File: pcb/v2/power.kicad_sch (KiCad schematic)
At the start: 72 parts, among them J16 TestPoint, J17 TestPoint, J4 Conn_01x02, J5 TestPoint, J6 TestPoint, J7 Conn_01x02, J8 Conn_01x02, J9 TestPoint, Q1 NPN, Q2 PMOS, U15 LP5907MFX-3.3, U2 TPS61230DRC, U3 LM27762, U4 TLV6213x, U5 BQ25895RTW

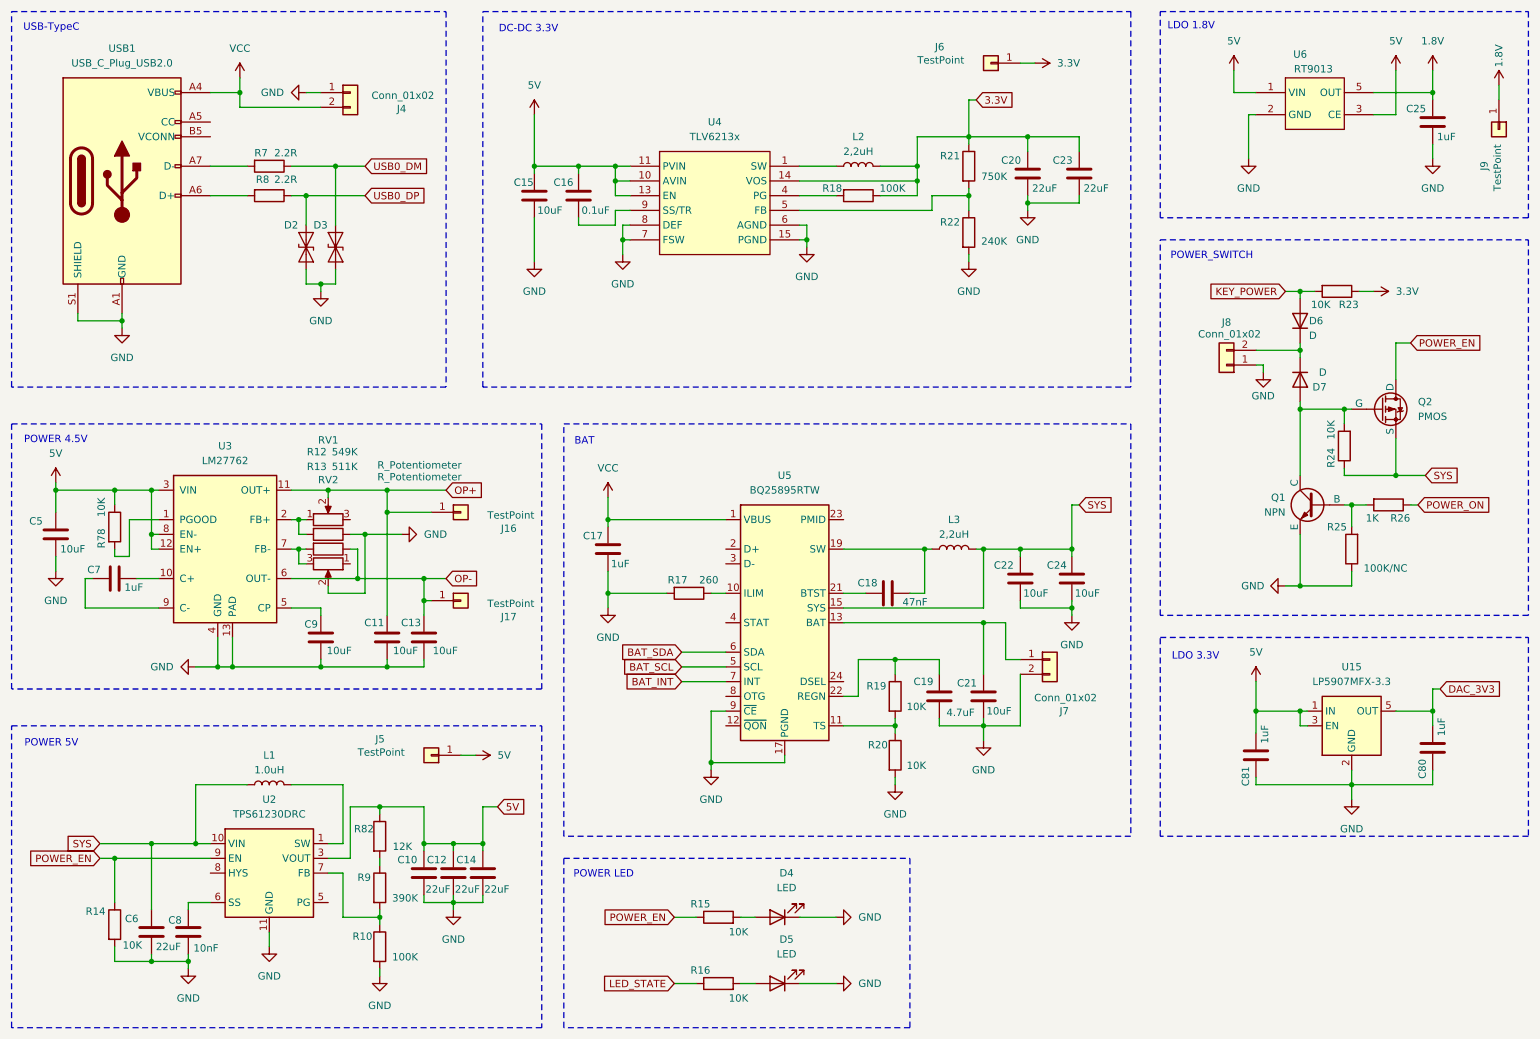
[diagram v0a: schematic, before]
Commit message: up
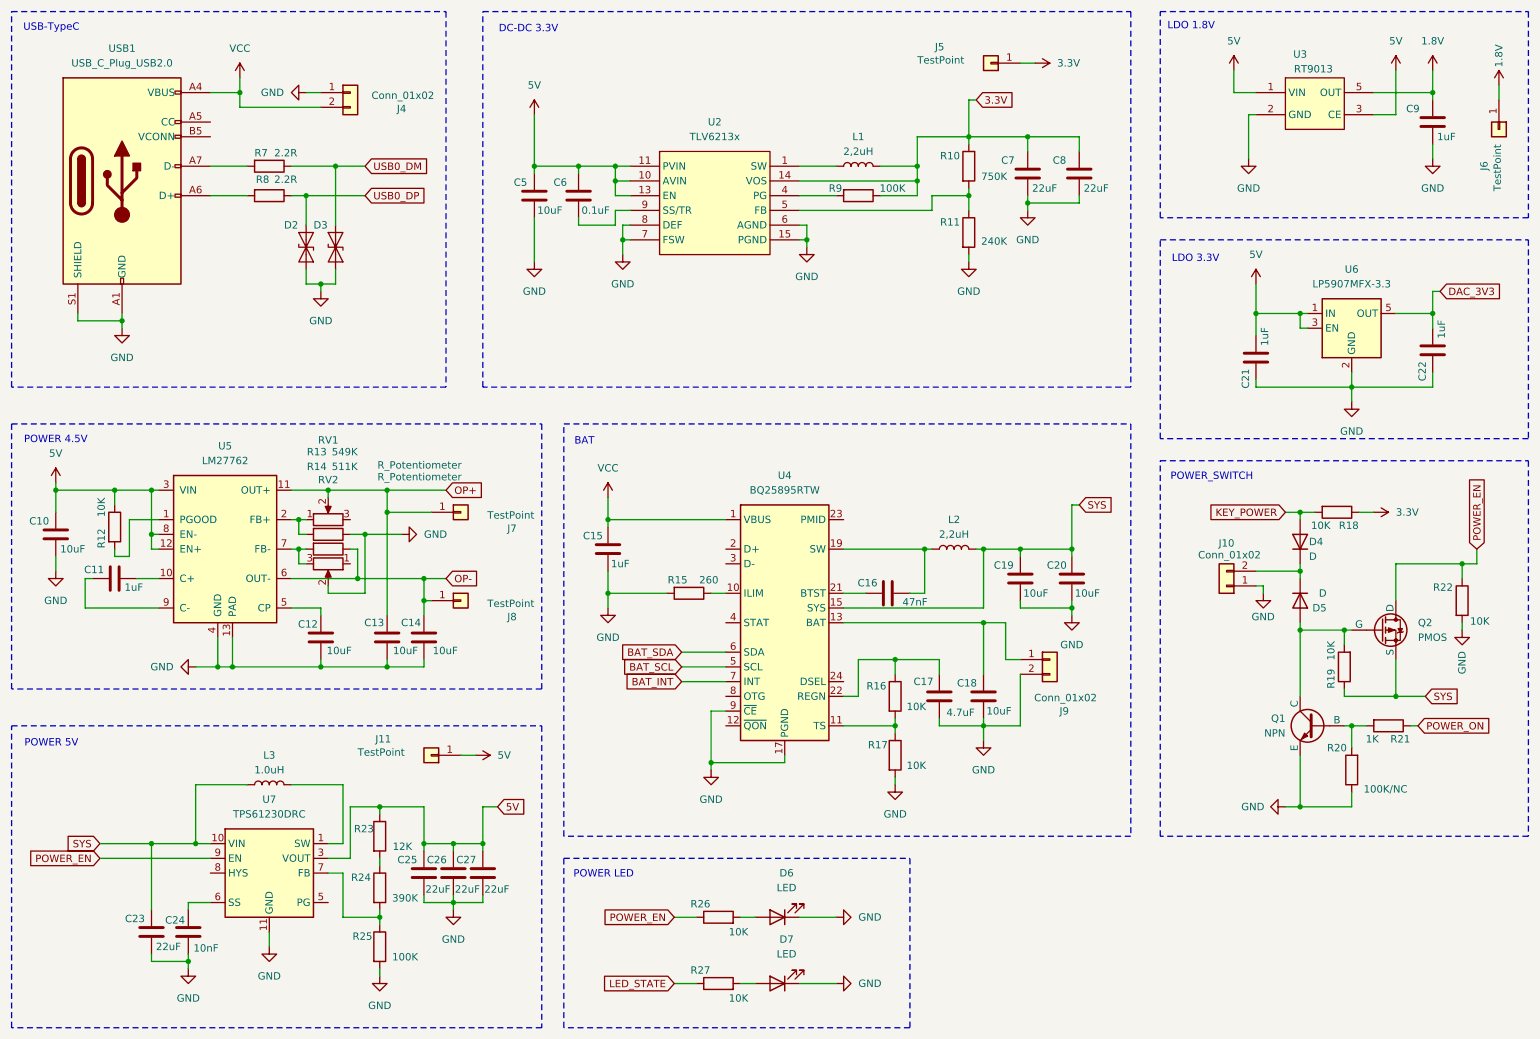
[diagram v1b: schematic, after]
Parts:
- renumbered C5 to C10, C7 to C11, C9 to C12, C11 to C13, C13 to C14, C17 to C15, C18 to C16, C19 to C17, C21 to C18, C22 to C19, C24 to C20, C81 to C21, C80 to C22, C6 to C23, C8 to C24, C10 to C25, C12 to C26, C14 to C27, C15 to C5, C16 to C6, C20 to C7, C23 to C8, C25 to C9, D6 to D4, D7 to D5, D4 to D6, D5 to D7, J8 to J10, J5 to J11, J6 to J5, J9 to J6, J16 to J7, J17 to J8, J7 to J9, L2 to L1, L3 to L2, L1 to L3, R21 to R10, R22 to R11, R78 to R12, R12 to R13, R13 to R14, R17 to R15, R19 to R16, R20 to R17, R23 to R18, R24 to R19, R25 to R20, R26 to R21, R14 to R22, R82 to R23, R9 to R24, R10 to R25, R15 to R26, R16 to R27, R18 to R9, U4 to U2, U6 to U3, U5 to U4, U3 to U5, U15 to U6, U2 to U7
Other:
- moved on the sheet: C21, C22, D4, D5, J10, Q1, Q2, R18, R19, R20, R21, R22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

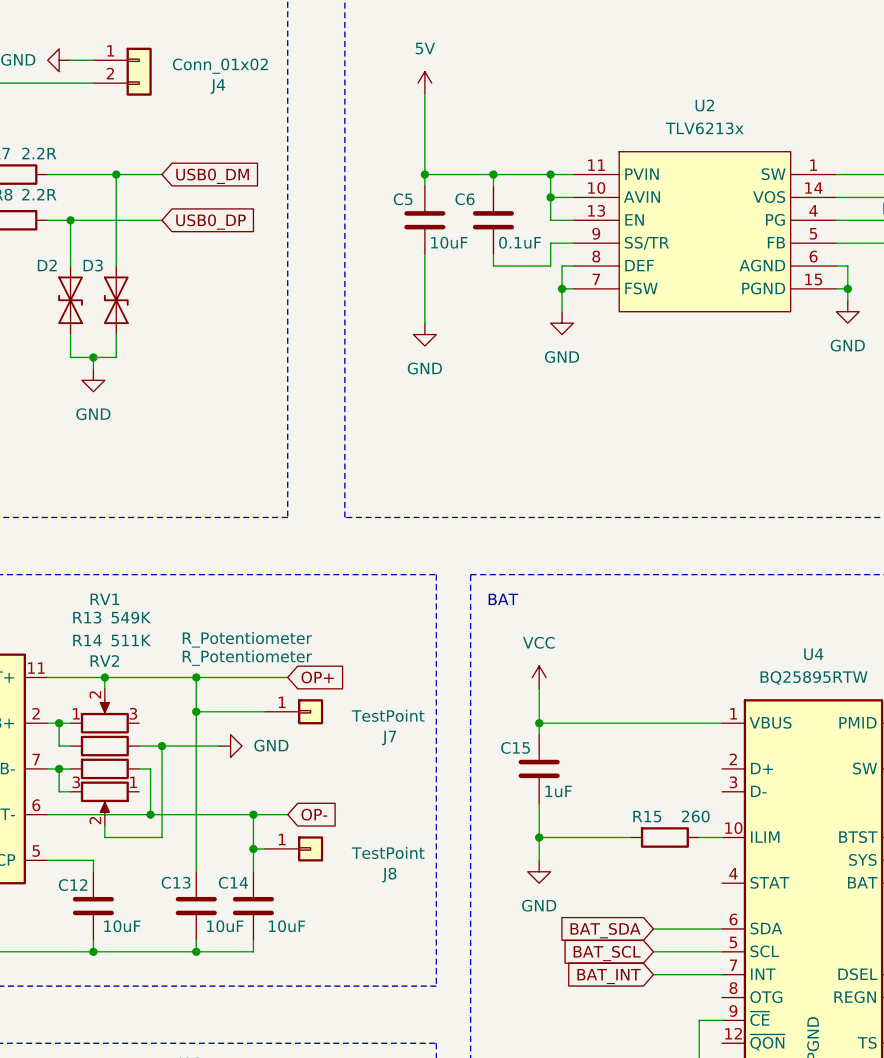
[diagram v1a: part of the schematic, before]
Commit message: up
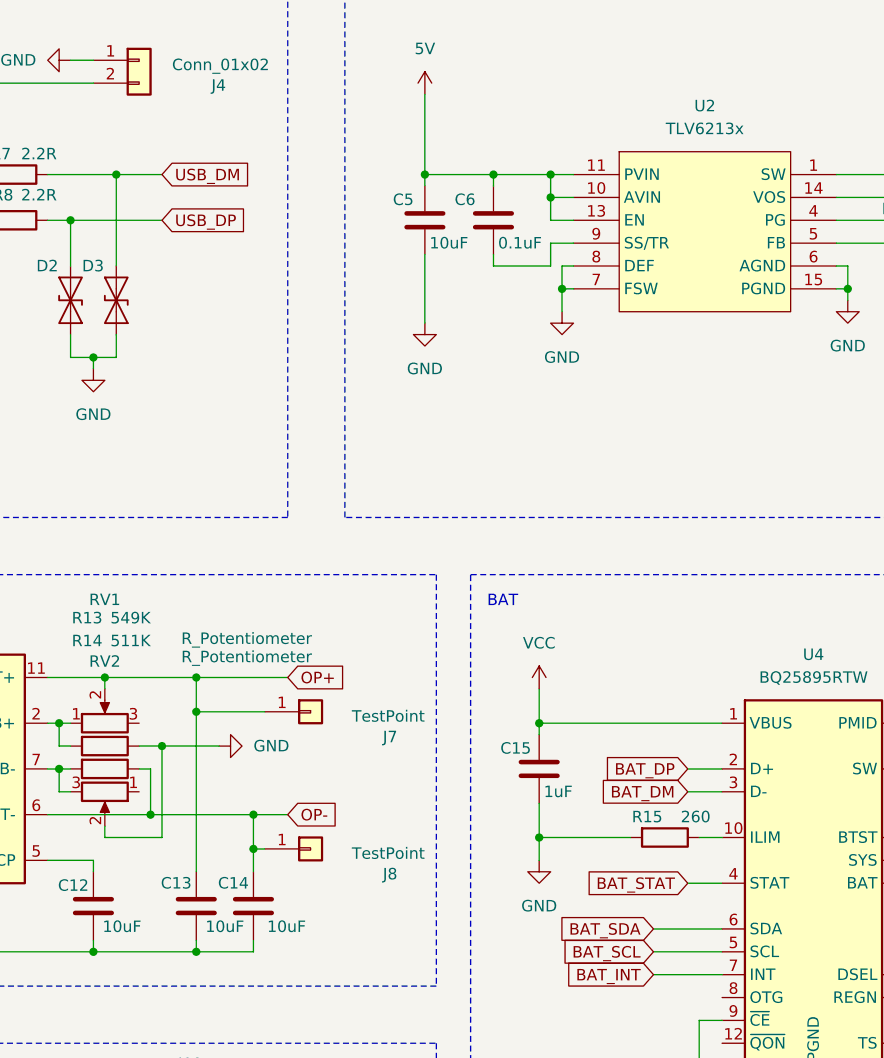
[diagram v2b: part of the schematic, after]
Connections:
- net BAT_DP: now reaches U4.2 (D+)
- net BAT_DM: now reaches U4.3 (D-)
- net BAT_STAT: now reaches U4.4 (STAT)
- net USB0_DM renamed USB_DM
- net USB0_DP renamed USB_DP
